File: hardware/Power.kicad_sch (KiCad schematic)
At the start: 10 parts, among them J8 USB_C_Receptacle_USB2.0_16P

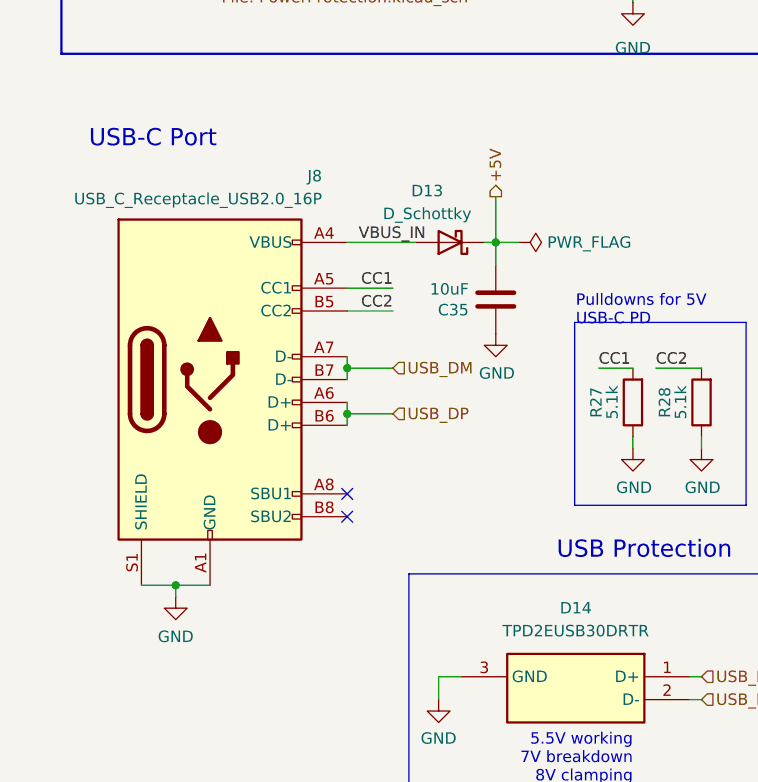
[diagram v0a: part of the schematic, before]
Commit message: fixed ERC, made it look pretty
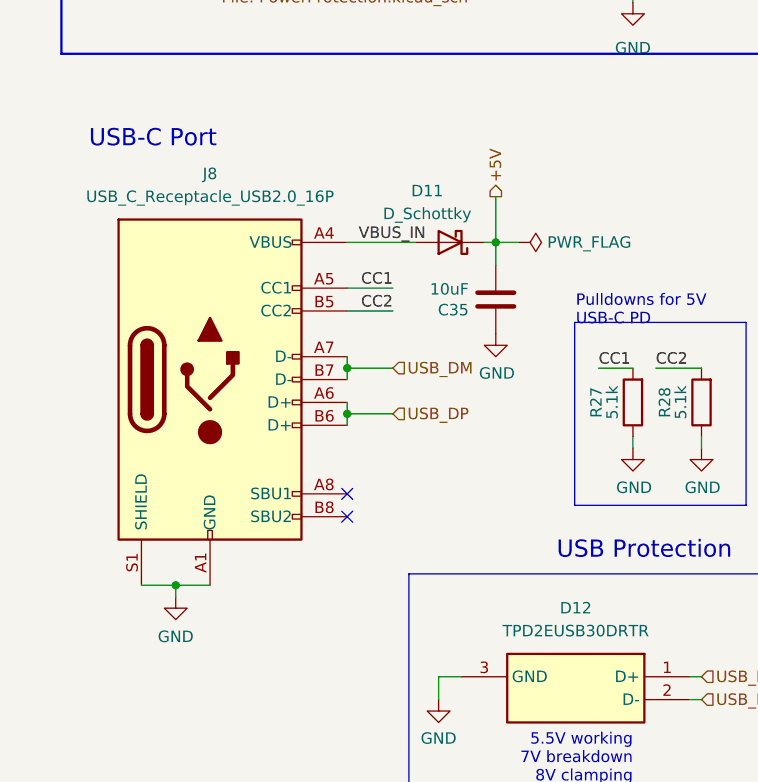
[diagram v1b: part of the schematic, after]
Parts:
- removed D14: TPD2EUSB30DRTR, LHRS_ICs:TPD2EUSB30DRTR, symbol USB_PD_Symbols:TPD2EUSB30DRTR
- removed J8: USB_C_Receptacle_USB2.0_16P, LHRS_Connectors:USB_C_Receptacle_GCT_USB4105-xx-A_16P_TopMnt_Horizontal, symbol UTSVT-Connectors:USB_C_Receptacle_USB2.0_16P
- added D12: TPD2EUSB30DRTR, LHRS_ICs:TPD2EUSB30DRTR, symbol lhrs_ics:TPD2EUSB30DRTR
- added J8: USB_C_Receptacle_USB2.0_16P, LHRS_Connectors:USB_C_Receptacle_GCT_USB4105-xx-A_16P_TopMnt_Horizontal, symbol lhrs_connectors:USB_C_Receptacle_USB2.0_16P
- TP13, TP14, TP15, TP16: footprint (none) -> LHRS_Special:TestPoint_HEX_3mmID
- renumbered D13 to D11
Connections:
- net CC1: now also J8.A5 (CC1)
- net CC2: now also J8.B5 (CC2)
- net GND: now also D12.3 (GND), J8.A1 (GND), J8.A12 (GND), J8.B1 (GND), J8.B12 (GND), J8.S1 (SHIELD), J8.S2 (Shield), J8.S3 (Shield), J8.S4 (Shield)
- net USB_DM: now also D12.2 (D-), J8.A7 (D-), J8.B7 (D-)
- net USB_DP: now also D12.1 (D+), J8.A6 (D+), J8.B6 (D+)
- net VBUS_IN: now also J8.A4 (VBUS), J8.A9 (VBUS), J8.B4 (VBUS), J8.B9 (VBUS)
